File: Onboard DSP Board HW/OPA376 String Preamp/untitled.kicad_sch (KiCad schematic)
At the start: 11 parts, among them J1 Input, U1 OPA376AIDCKT

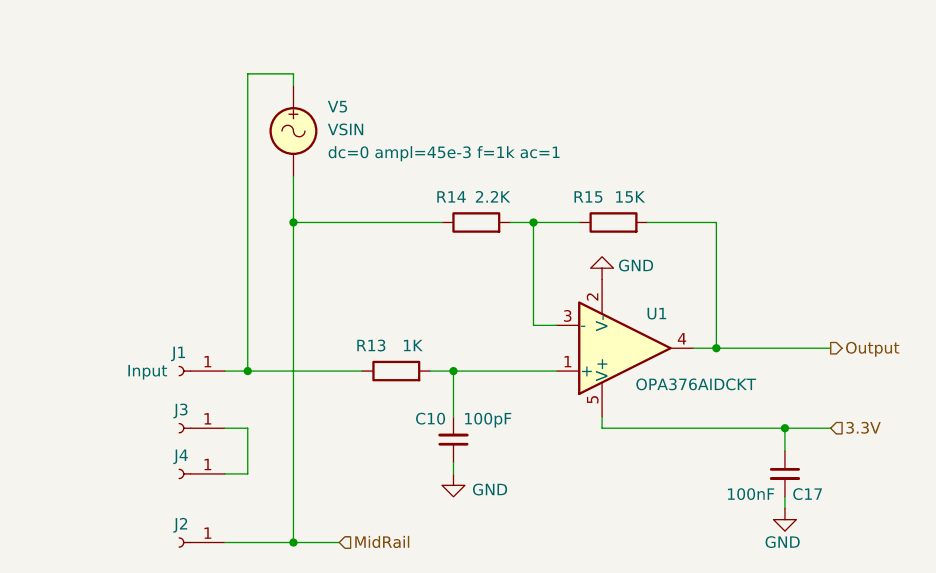
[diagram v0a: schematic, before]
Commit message: WIP
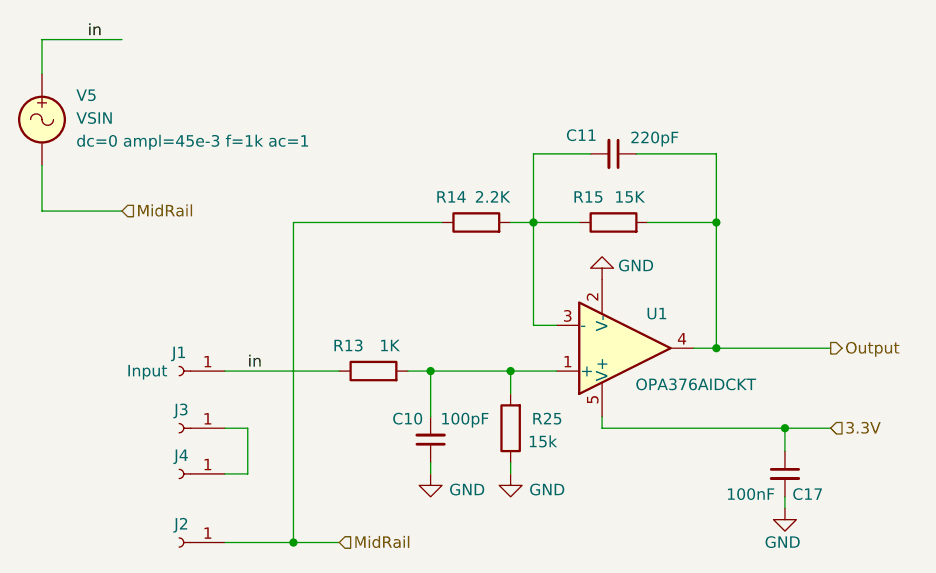
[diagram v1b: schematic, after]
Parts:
- added C11: 220pF, Capacitor_SMD:C_0402_1005Metric, symbol Device:C_Small
- added R25: 15k, Resistor_SMD:R_0402_1005Metric, symbol Device:R
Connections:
- net GND: now also R25.1
- net Output: now also C11.1
- net in: now reaches J1.1 (Pin_1), R13.1, V5.1
- net at C10.2, R13.2, U1.1 (+): now also R25.2
- net at R14.2, R15.1, U1.3 (-): now also C11.2
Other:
- moved on the sheet: C10, R13, V5
